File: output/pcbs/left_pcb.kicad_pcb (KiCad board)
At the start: 2 copper layers, 132 x 117.7 mm, 37 parts

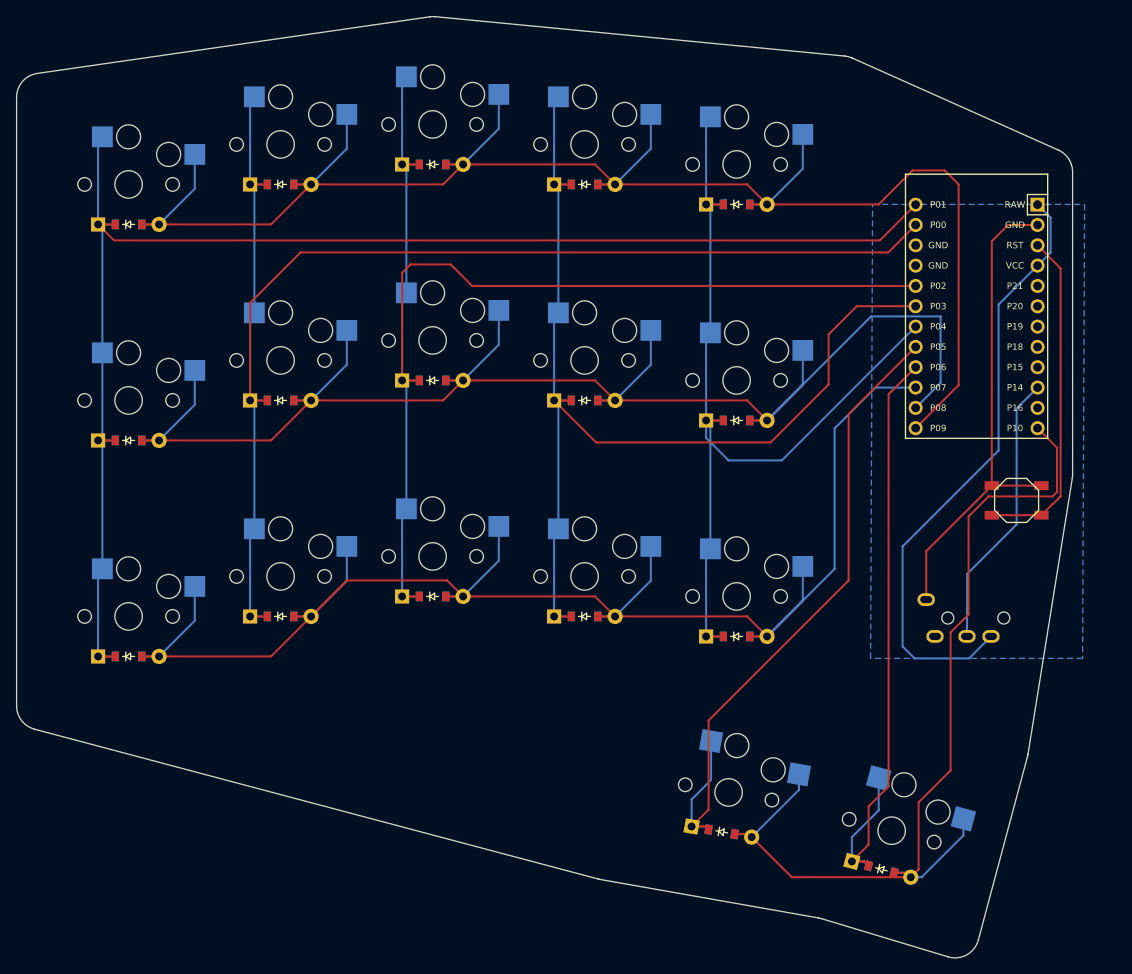
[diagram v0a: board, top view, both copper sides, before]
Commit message: fix spacing
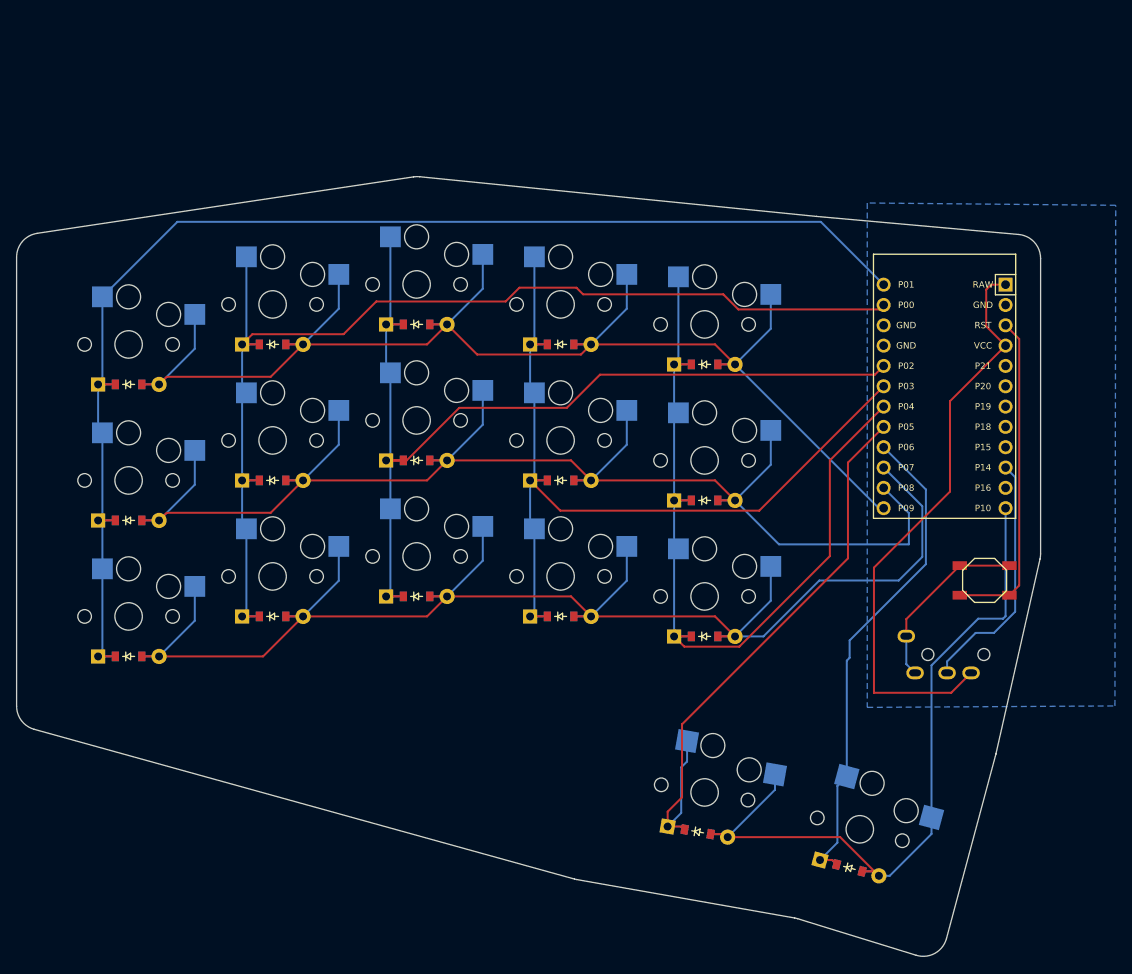
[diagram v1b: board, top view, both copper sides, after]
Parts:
- moved D15 20.4 mm to (172.0, 68.5)
- moved S15 20.4 mm to (172.0, 63.5)
- moved D12 20.2 mm to (154.0, 66.0)
- moved S12 20.2 mm to (154.0, 61.0)
- moved D9 20.1 mm to (136.0, 63.5)
- moved S9 20.1 mm to (136.0, 58.5)
- moved D6 20.0 mm to (118.0, 66.0)
- moved S6 20.0 mm to (118.0, 61.0)
- moved D3 20.0 mm to (100.0, 71.0)
- moved S3 20.0 mm to (100.0, 66.0)
- moved B1 10.8 mm to (207.0, 95.5)
- moved D14 10.8 mm to (172.0, 85.5)
- moved MCU1 10.8 mm to (202.0, 72.5)
- moved S14 10.8 mm to (172.0, 80.5)
- moved D11 10.4 mm to (154.0, 83.0)
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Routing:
- net GND: track 61.0 -> 22.8 mm
- net L_R2: track 214.9 -> 178.8 mm
- net L_C1: track 178.4 -> 143.5 mm
- net L_C2: track 158.2 -> 126.1 mm
- net L_R3: track 121.7 -> 95.5 mm
- net L_C3: track 137.1 -> 111.2 mm
- net L_C0: track 183.9 -> 163.8 mm
- net L_T1: track 81.5 -> 63.9 mm
- net L_R1: track 195.6 -> 184.1 mm
- net L_C4: track 116.0 -> 105.2 mm
- net L_T0: track 87.8 -> 77.4 mm
- net L_R0: track 199.2 -> 192.5 mm
- net SERIAL: track 34.8 -> 31.0 mm
- net VCC: track 76.4 -> 74.1 mm
- net RST: track 42.2 -> 41.2 mm
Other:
- board size 132 x 117.7 mm -> 128 x 97.5 mm
